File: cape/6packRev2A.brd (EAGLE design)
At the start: 38.1 x 209.2 mm, 16 parts

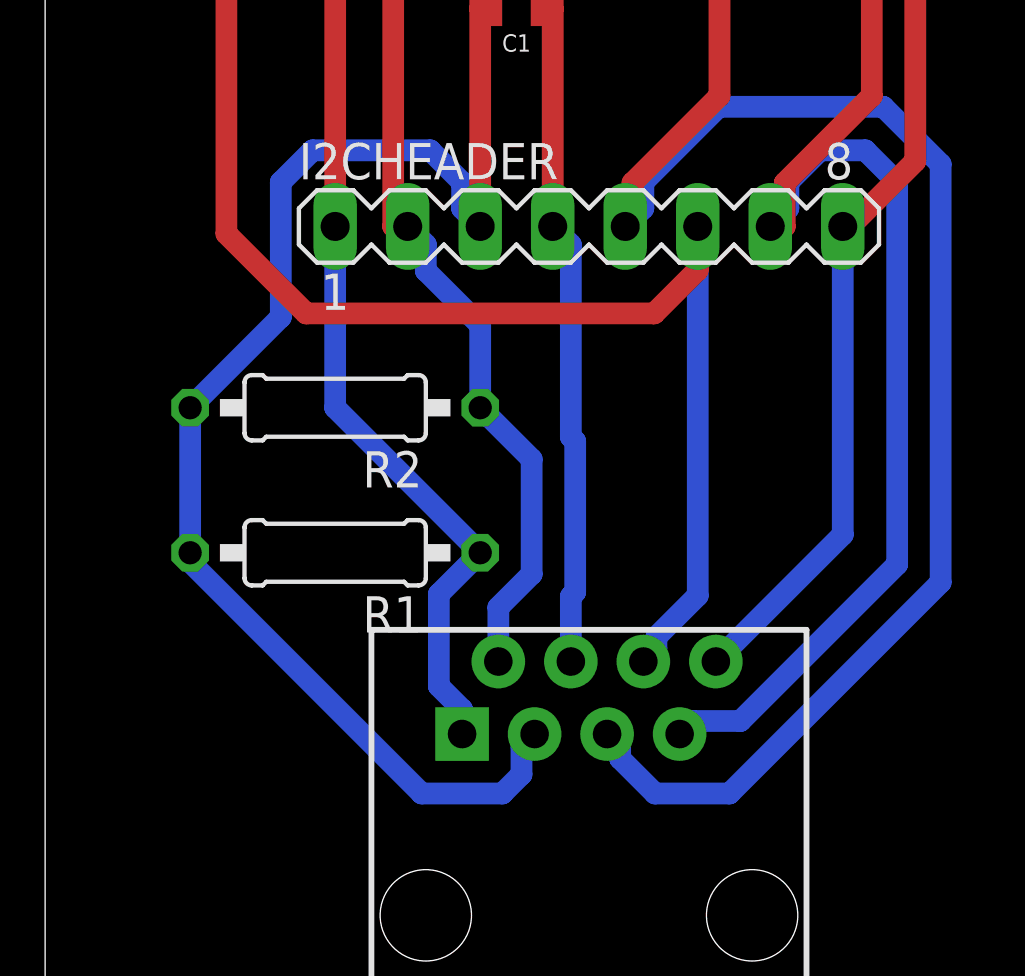
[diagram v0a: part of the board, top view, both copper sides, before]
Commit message: Revert "Update 6Pack 2A"
This reverts commit 827b5304b12bda17fe1987ea76be93996f945791.
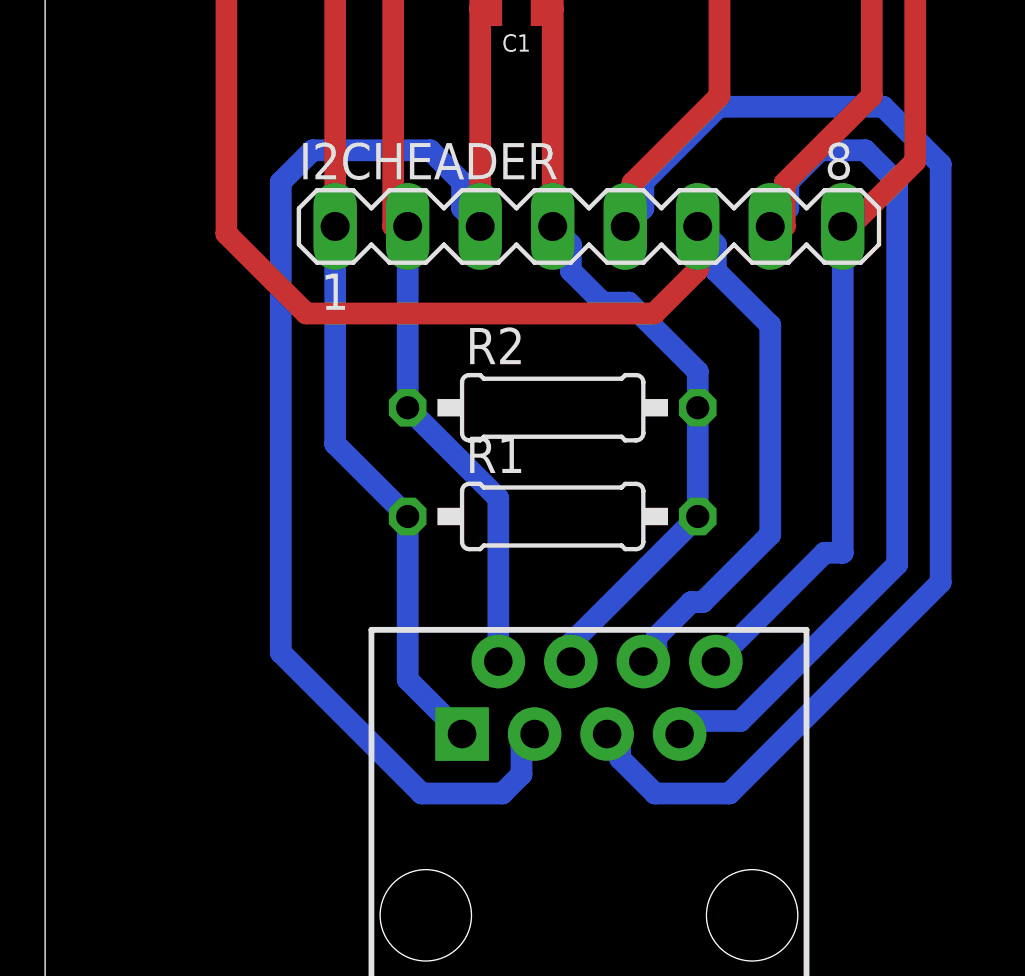
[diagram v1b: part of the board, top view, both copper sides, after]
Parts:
- moved R1 7.73 mm to (17.8, 24.1), turned to 0 degrees
- moved R2 7.62 mm to (17.8, 27.9), turned to 0 degrees
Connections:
- net +5V1: no longer R1.2, R2.2
- net GND1: now also R1.2, R2.2
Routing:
- net GND1: track 196.1 -> 200.2 mm
- net +5V1: track 258.3 -> 255.7 mm
- net +5V2: track 197.6 -> 200.0 mm
- net SCL1: track 201.8 -> 200.6 mm
- net SDA1: track 197.8 -> 196.8 mm
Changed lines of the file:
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@@
 <attribute name="VALUE" x="16.672" y="161.128" size="1.27" layer="27"/>
 </element>
-<element name="R1" library="resistor" library_urn="urn:adsk.eagle:library:348" package="0207/10" package3d_urn="urn:adsk.eagle:package:25939/1" value="4.7kΩ" x="10.16" y="22.86" rot="R180">
-<attribute name="NAME" x="13.208" y="21.336" size="1.27" layer="25" ratio="10" rot="R180"/>
-<attribute name="VALUE" x="12.4206" y="23.495" size="1.27" layer="27" ratio="10" rot="R180"/>
+<element name="R1" library="resistor" library_urn="urn:adsk.eagle:library:348" package="0207/10" package3d_urn="urn:adsk.eagle:package:25939/1" value="4.7kΩ" x="17.78" y="24.13">
+<attribute name="NAME" x="14.732" y="25.654" size="1.27" layer="25" ratio="10"/>
+<attribute name="VALUE" x="15.5194" y="23.495" size="1.27" layer="27" ratio="10"/>
 </element>
-<element name="R2" library="resistor" library_urn="urn:adsk.eagle:library:348" package="0207/10" package3d_urn="urn:adsk.eagle:package:25939/1" value="4.7kΩ" x="10.16" y="27.94" rot="R180">
-<attribute name="NAME" x="13.208" y="26.416" size="1.27" layer="25" ratio="10" rot="R180"/>
-<attribute name="VALUE" x="12.4206" y="28.575" size="1.27" layer="27" ratio="10" rot="R180"/>
+<element name="R2" library="resistor" library_urn="urn:adsk.eagle:library:348" package="0207/10" package3d_urn="urn:adsk.eagle:package:25939/1" value="4.7kΩ" x="17.78" y="27.94">
+<attribute name="NAME" x="14.732" y="29.464" size="1.27" layer="25" ratio="10"/>
+<attribute name="VALUE" x="15.5194" y="27.305" size="1.27" layer="27" ratio="10"/>
 </element>
 </elements>
@@
 <wire x1="16.6878" y1="15.09675625" x2="16.01824375" y2="14.4272" width="0.762" layer="16"/>
 <wire x1="16.01824375" y1="14.4272" x2="13.19175625" y2="14.4272" width="0.762" layer="16"/>
-<wire x1="17.145" y1="16.51" x2="16.6878" y2="16.0528" width="0.762" layer="16"/>
-<wire x1="16.6878" y1="16.0528" x2="16.6878" y2="15.09675625" width="0.762" layer="16"/>
-<contactref element="R2" pad="2"/>
-<contactref element="R1" pad="2"/>
-<wire x1="13.19175625" y1="14.4272" x2="5.08" y2="22.53895625" width="0.762" layer="16"/>
-<wire x1="5.08" y1="22.53895625" x2="5.08" y2="22.86" width="0.762" layer="16"/>
-<wire x1="5.08" y1="22.86" x2="5.08" y2="27.94" width="0.762" layer="16"/>
 <wire x1="8.255" y1="35.84108125" x2="9.37091875" y2="36.957" width="0.762" layer="16"/>
 <wire x1="13.48908125" y1="36.957" x2="14.605" y2="35.84108125" width="0.762" layer="16"/>
 <wire x1="9.37091875" y1="36.957" x2="13.48908125" y2="36.957" width="0.762" layer="16"/>
-<wire x1="5.08" y1="27.94" x2="8.255" y2="31.115" width="0.762" layer="16"/>
 <wire x1="14.605" y1="35.84108125" x2="14.605" y2="34.925" width="0.762" layer="16"/>
 <wire x1="14.605" y1="34.925" x2="15.24" y2="34.29" width="0.762" layer="16"/>
-<wire x1="8.255" y1="31.115" x2="8.255" y2="35.84108125" width="0.762" layer="16"/>
+<wire x1="17.145" y1="16.51" x2="16.6878" y2="16.0528" width="0.762" layer="16"/>
+<wire x1="16.6878" y1="16.0528" x2="16.6878" y2="15.09675625" width="0.762" layer="16"/>
+<wire x1="13.19175625" y1="14.4272" x2="8.255" y2="19.36395625" width="0.762" layer="16"/>
+<wire x1="8.255" y1="19.36395625" x2="8.255" y2="35.84108125" width="0.762" layer="16"/>
 </signal>
 <signal name="GND1">
@@
 <wire x1="11.43" y1="155.448" x2="7.62" y2="159.258" width="0.762" layer="1"/>
 <wire x1="11.43" y1="155.448" x2="11.43" y2="154.94" width="0.762" layer="1"/>
+<contactref element="R1" pad="2"/>
+<contactref element="R2" pad="2"/>
+<wire x1="18.415" y1="19.05" x2="18.415" y2="19.685" width="0.762" layer="16"/>
+<wire x1="18.415" y1="19.685" x2="22.86" y2="24.13" width="0.762" layer="16"/>
+<wire x1="22.86" y1="24.13" x2="22.86" y2="27.94" width="0.762" layer="16"/>
+<wire x1="22.86" y1="27.94" x2="22.86" y2="29.21" width="0.762" layer="16"/>
+<wire x1="22.86" y1="29.21" x2="20.447" y2="31.623" width="0.762" layer="16"/>
+<wire x1="20.447" y1="31.623" x2="19.53091875" y2="31.623" width="0.762" layer="16"/>
+<wire x1="19.53091875" y1="31.623" x2="18.415" y2="32.73891875" width="0.762" layer="16"/>
+<wire x1="18.415" y1="32.73891875" x2="18.415" y2="33.655" width="0.762" layer="16"/>
+<wire x1="18.415" y1="33.655" x2="17.78" y2="34.29" width="0.762" layer="16"/>
 <wire x1="11.43" y1="175.26" x2="19.05" y2="182.88" width="0.762" layer="1"/>
 <via x="19.05" y="182.88" extent="1-16" drill="0.65" diameter="1.3"/>
@@
 <wire x1="19.2278" y1="189.637275" x2="19.2278" y2="190.0428" width="0.762" layer="16"/>
 <wire x1="19.2278" y1="190.0428" x2="19.685" y2="190.5" width="0.762" layer="16"/>
-<wire x1="18.415" y1="33.655" x2="17.78" y2="34.29" width="0.762" layer="16"/>
-<wire x1="18.415" y1="19.05" x2="18.415" y2="21.32934375" width="0.762" layer="16"/>
-<wire x1="18.415" y1="21.32934375" x2="18.5674" y2="21.48174375" width="0.762" layer="16"/>
-<wire x1="18.5674" y1="21.48174375" x2="18.5674" y2="26.7678625" width="0.762" layer="16"/>
-<wire x1="18.5674" y1="26.7678625" x2="18.415" y2="26.9202625" width="0.762" layer="16"/>
-<wire x1="18.415" y1="26.9202625" x2="18.415" y2="33.655" width="0.762" layer="16"/>
 </signal>
 <signal name="SCL1">
@@
 <wire x1="24.3078" y1="180.103875" x2="24.3078" y2="191.362725" width="0.762" layer="16"/>
 <contactref element="R1" pad="1"/>
+<wire x1="14.605" y1="16.51" x2="12.7" y2="18.415" width="0.762" layer="16"/>
+<wire x1="12.7" y1="24.13" x2="12.7" y2="18.415" width="0.762" layer="16"/>
+<wire x1="12.7" y1="24.13" x2="10.16" y2="26.67" width="0.762" layer="16"/>
+<wire x1="10.16" y1="26.67" x2="10.16" y2="34.29" width="0.762" layer="16"/>
 <via x="10.16" y="44.45" extent="1-16" drill="0.65" diameter="1.3"/>
 <wire x1="10.16" y1="50.038" x2="10.16" y2="44.45" width="0.762" layer="16"/>
 <wire x1="10.16" y1="44.45" x2="10.16" y2="34.29" width="0.762" layer="1"/>
-<wire x1="15.24" y1="22.86" x2="10.16" y2="27.94" width="0.762" layer="16"/>
-<wire x1="10.16" y1="27.94" x2="10.16" y2="34.29" width="0.762" layer="16"/>
-<wire x1="14.605" y1="16.51" x2="14.605" y2="17.374475" width="0.762" layer="16"/>
-<wire x1="14.605" y1="17.374475" x2="13.7922" y2="18.187275" width="0.762" layer="16"/>
-<wire x1="13.7922" y1="18.187275" x2="13.7922" y2="21.4122" width="0.762" layer="16"/>
-<wire x1="13.7922" y1="21.4122" x2="15.24" y2="22.86" width="0.762" layer="16"/>
 </signal>
 <signal name="SDA1">
@@
 <wire x1="22.225" y1="180.561075" x2="22.225" y2="190.5" width="0.762" layer="16"/>
 <contactref element="R2" pad="1"/>
-<wire x1="15.875" y1="19.05" x2="15.875" y2="20.94460625" width="0.762" layer="16"/>
-<wire x1="15.875" y1="20.94460625" x2="17.0434" y2="22.11300625" width="0.762" layer="16"/>
-<wire x1="17.0434" y1="22.11300625" x2="17.0434" y2="26.1366" width="0.762" layer="16"/>
-<wire x1="17.0434" y1="26.1366" x2="15.24" y2="27.94" width="0.762" layer="16"/>
-<wire x1="13.335" y1="32.73891875" x2="13.335" y2="33.655" width="0.762" layer="16"/>
-<wire x1="13.335" y1="33.655" x2="12.7" y2="34.29" width="0.762" layer="16"/>
-<wire x1="15.24" y1="27.94" x2="15.24" y2="30.83391875" width="0.762" layer="16"/>
-<wire x1="15.24" y1="30.83391875" x2="13.335" y2="32.73891875" width="0.762" layer="16"/>
+<wire x1="15.875" y1="19.05" x2="15.875" y2="24.765" width="0.762" layer="16"/>
+<wire x1="15.875" y1="24.765" x2="12.7" y2="27.94" width="0.762" layer="16"/>
+<wire x1="12.7" y1="27.94" x2="12.7" y2="34.29" width="0.762" layer="16"/>
 </signal>
 <signal name="GND2">
@@
 <wire x1="6.35" y1="34.036" x2="6.35" y2="73.0287375" width="0.762" layer="1"/>
 <wire x1="17.145" y1="190.5" x2="17.145" y2="183.515" width="0.762" layer="16"/>
+<wire x1="20.955" y1="19.05" x2="21.4122" y2="19.5072" width="0.762" layer="16"/>
+<wire x1="21.4122" y1="19.5072" x2="21.4122" y2="19.912725" width="0.762" layer="16"/>
+<wire x1="21.4122" y1="19.912725" x2="22.632275" y2="21.1328" width="0.762" layer="16"/>
+<wire x1="22.632275" y1="21.1328" x2="23.0378" y2="21.1328" width="0.762" layer="16"/>
+<wire x1="23.0378" y1="21.1328" x2="25.4" y2="23.495" width="0.762" layer="16"/>
+<wire x1="23.495" y1="32.73891875" x2="23.495" y2="33.655" width="0.762" layer="16"/>
+<wire x1="23.495" y1="33.655" x2="22.86" y2="34.29" width="0.762" layer="16"/>
+<wire x1="25.4" y1="30.83391875" x2="23.495" y2="32.73891875" width="0.762" layer="16"/>
+<wire x1="25.4" y1="23.495" x2="25.4" y2="30.83391875" width="0.762" layer="16"/>
 <wire x1="17.145" y1="183.515" x2="16.51" y2="182.88" width="0.762" layer="16"/>
 <via x="16.51" y="182.88" extent="1-16" drill="0.65" diameter="1.3"/>
 <wire x1="16.51" y1="182.88" x2="10.587" y2="176.957" width="0.762" layer="1"/>
-<wire x1="20.955" y1="19.05" x2="21.4122" y2="19.5072" width="0.762" layer="16"/>
-<wire x1="21.4122" y1="19.5072" x2="21.4122" y2="19.912725" width="0.762" layer="16"/>
-<wire x1="22.86" y1="21.360525" x2="22.86" y2="34.29" width="0.762" layer="16"/>
-<wire x1="21.4122" y1="19.912725" x2="22.86" y2="21.360525" width="0.762" layer="16"/>
 </signal>
 <signal name="SDA2">
@@
 <wire x1="28.194" y1="34.29" x2="30.48" y2="36.576" width="0.762" layer="1"/>
 <wire x1="28.194" y1="34.29" x2="27.94" y2="34.29" width="0.762" layer="1"/>
+<wire x1="23.495" y1="19.05" x2="27.305" y2="22.86" width="0.762" layer="16"/>
+<wire x1="27.305" y1="22.86" x2="27.94" y2="22.86" width="0.762" layer="16"/>
+<wire x1="27.94" y1="22.86" x2="27.94" y2="34.29" width="0.762" layer="16"/>
 <wire x1="21.336" y1="188.214" x2="15.464" y2="188.214" width="0.762" layer="1"/>
 <wire x1="15.464" y1="188.214" x2="15.352" y2="188.102" width="0.762" layer="1"/>
@@
 <wire x1="15.352" y1="188.102" x2="14.605" y2="188.849" width="0.762" layer="16"/>
 <wire x1="14.605" y1="188.849" x2="14.605" y2="190.5" width="0.762" layer="16"/>
-<wire x1="23.495" y1="19.05" x2="27.94" y2="23.495" width="0.762" layer="16"/>
-<wire x1="27.94" y1="23.495" x2="27.94" y2="34.29" width="0.762" layer="16"/>
 </signal>
 </signals>
